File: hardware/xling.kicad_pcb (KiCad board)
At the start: 2 copper layers, 45 x 60 mm, 57 parts, among them J3 MCP73831, J4 USB_OTG, J5 AVR ISP, J6 Battery, Q1 TP0610T, SW2 Up, SW3 Select, SW4 Down, U1 LT1109CZ-12, U2 ATMEGA328P-AU, U3 DEP_128064I, U4 MCP1640B-CH, U5 LM1117-3.3, Y1 8MHz

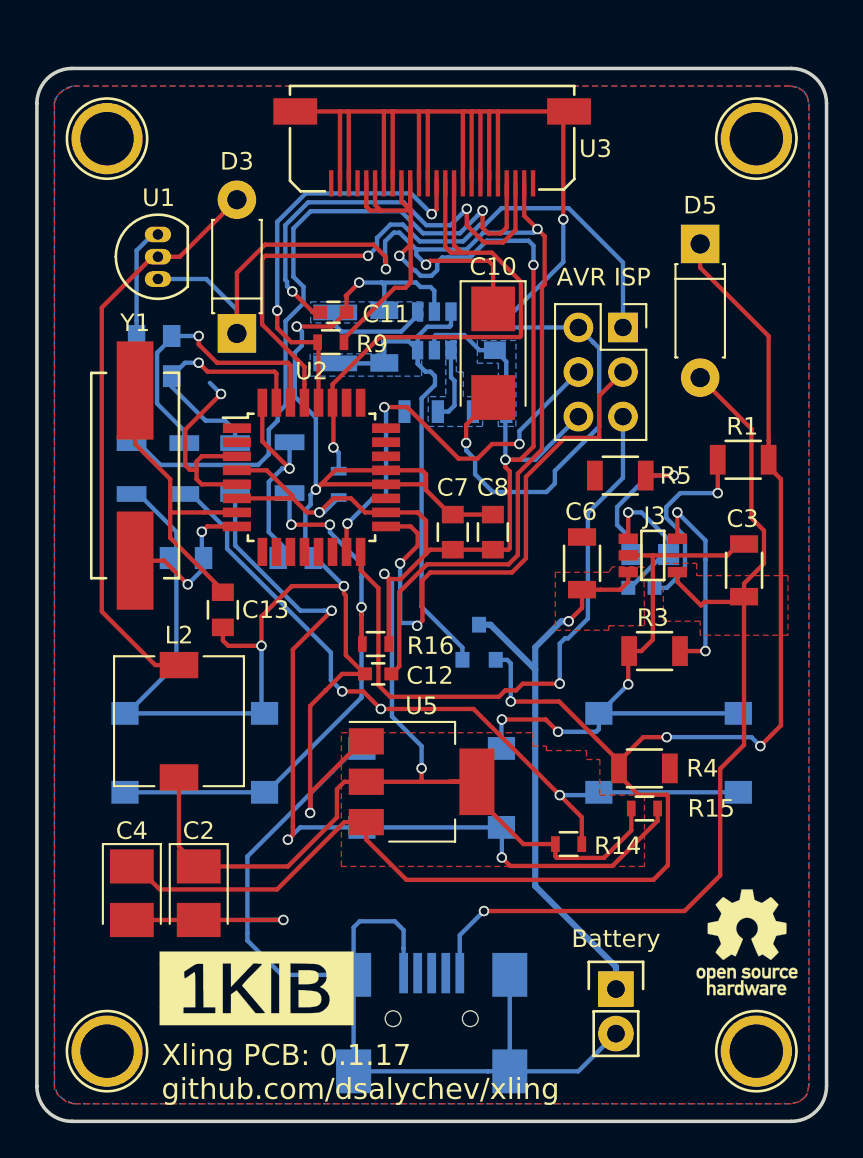
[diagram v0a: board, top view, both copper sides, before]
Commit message: patch 0.1.18: Add new KiCad modules and scheme changes.
Signed-off-by: Dmitry Salychev <darkness.bsd@gmail.com>
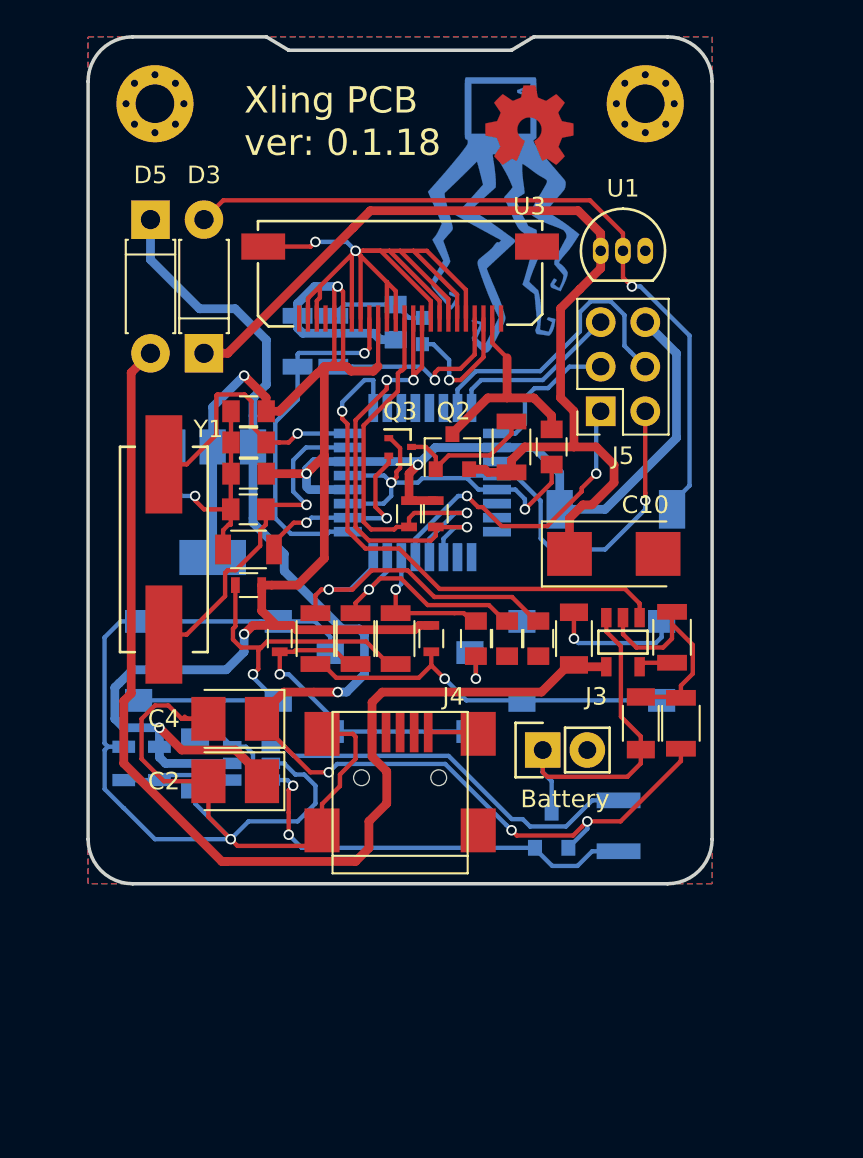
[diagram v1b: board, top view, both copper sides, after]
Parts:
- removed C12: 2.2uF, Capacitors_SMD:C_0603
- removed D1: charging, LEDs:LED_0603
- removed D2: charged, LEDs:LED_0805
- removed the G*** at (131.5, 130.4)
- removed the REF** at (160.0, 134.0)
- removed the REF** at (123.0, 134.0)
- removed the REF** at (160.0, 82.0)
- removed the REF** at (123.0, 82.0)
- removed REF***: OSHW-Logo_5.7x6mm_SilkScreen, Symbols:OSHW-Logo_5.7x6mm_SilkScreen
- added C9: 1pF, Capacitors_SMD:C_0805, F.Cu at (148.3, 99.6)
- added G***: LOGO, Xling Footprints:terterm, B.Cu at (145.5, 86.4)
- added G***: LOGO, Xling Footprints:oshw, F.Cu at (147.1, 81.3)
- added Q2: NTR0202PL, TO_SOT_Packages_SMD:SOT-23, F.Cu at (142.7, 99.8)
- added Q3: NTA4153N, SC-75_SOT-416, F.Cu at (139.7, 99.6)
- added R10: 100K, Resistors_SMD:R_1206, F.Cu at (131.1, 105.4)
- added REF**: MountingHole_2.2mm_M2_Pad_Via, Mounting_Holes:MountingHole_2.2mm_M2_Pad_Via, F.Cu at (125.7, 80.0)
- added REF**: MountingHole_2.2mm_M2_Pad_Via, Mounting_Holes:MountingHole_2.2mm_M2_Pad_Via, F.Cu at (153.7, 80.0)
- C11, L2, U2: moved to B.Cu
- C15, C18, C19, C20, J4, R17, R18, R19, R8: moved to F.Cu
- J6: footprint Pin_Headers:Pin_Header_Straight_1x02 -> Xling Footprints:Pin_Header_Straight_1x02
- R1: value 470R -> 100K; moved to B.Cu
- R5: value 470R -> 100K
- U5: footprint TO_SOT_Packages_SMD:SOT-223-3Lead_TabPin2 -> Xling Footprints:SOT-223-3Lead_TabPin2; moved to B.Cu
- Y1: footprint Crystals:Crystal_HC49-SD_SMD -> Xling Footprints:Crystal_HC49-SD_SMD
- moved L1 32.2 mm to (152.1, 121.2)
- moved D5 31.4 mm to (125.5, 86.6)
- moved L2 27.7 mm to (152.0, 103.1), turned to 0 degrees
- moved R6 27.5 mm to (126.0, 117.6), turned to 270 degrees
- moved U4 26.8 mm to (131.2, 117.6), turned to 180 degrees
- moved SW2 26.7 mm to (128.8, 111.8)
- moved C5 26.6 mm to (128.0, 117.6), turned to 270 degrees
- moved R1 26.3 mm to (133.9, 93.5), turned to 270 degrees
- moved R7 26.3 mm to (124.0, 117.6), turned to 90 degrees
- moved U1 25.3 mm to (151.1, 88.4), turned to 0 degrees
- moved C18 25.2 mm to (144.0, 110.5), turned to 270 degrees
- moved C19 25.1 mm to (145.8, 110.5), turned to 270 degrees
- moved R14 23.5 mm to (131.1, 107.4), turned to 180 degrees
- moved SW4 23.2 mm to (150.6, 111.8)
- moved R15 22.9 mm to (132.8, 110.5), turned to 270 degrees
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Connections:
- J3 pad 1: Net-(D1-Pad1) -> /BAT_STAT
- J4 pad 2: Net-(J4-Pad2) -> (no net)
- J4 pad 3: Net-(J4-Pad3) -> (no net)
- J4 pad 4: Net-(J4-Pad4) -> (no net)
- R1 pad 1: Net-(C4-Pad1) -> +3V3
- R1 pad 2: Net-(D1-Pad2) -> /OLED_RES
- R5 pad 1: GND -> +12V
- U2 pad 1: Net-(U2-Pad1) -> /OLED_RES
- U2 pad 10: Net-(U2-Pad10) -> (no net)
- U2 pad 11: Net-(U2-Pad11) -> (no net)
- U2 pad 12: Net-(U2-Pad12) -> (no net)
- U2 pad 13: Net-(U2-Pad13) -> (no net)
- U2 pad 14: Net-(U2-Pad14) -> (no net)
- U2 pad 19: Net-(U2-Pad19) -> (no net)
- U2 pad 2: Net-(U2-Pad2) -> /OLED_PWR
- U2 pad 22: Net-(U2-Pad22) -> (no net)
- U2 pad 23: Net-(U2-Pad23) -> (no net)
- U2 pad 24: Net-(U2-Pad24) -> (no net)
- U2 pad 25: Net-(U2-Pad25) -> (no net)
- U2 pad 26: Net-(U2-Pad26) -> (no net)
- U2 pad 9: Net-(U2-Pad9) -> /BAT_STAT
- U3 pad 1: Net-(U3-Pad1) -> (no net)
- U3 pad 23: +12V -> /OLED_VCC
- U3 pad 24: Net-(U3-Pad24) -> (no net)
- U3 pad 4: Net-(U3-Pad4) -> (no net)
- U3 pad 9: +3V3 -> /OLED_RES
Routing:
- net GND: track 328.7 -> 220.6 mm, vias 13 -> 9
- net Net-(R15-Pad2): track 49.3 -> 18.7 mm, vias 3 -> 1
- net /BAT_STAT: track 0.00 -> 30.5 mm, vias 0 -> 1
- net Net-(R2-Pad2): track 39.9 -> 11.3 mm
- net /ISP_PDO_MISO: track 35.7 -> 10.0 mm, vias 1 -> 0
- net /ISP_SCK: track 31.7 -> 8.35 mm, vias 2 -> 0
- net Net-(C4-Pad1): track 94.6 -> 72.3 mm, vias 3 -> 4
- net /OLED_RES: track 0.00 -> 20.4 mm, vias 0 -> 1
- net /ISP_RST: track 37.1 -> 18.1 mm, vias 1 -> 2
- net Net-(R14-Pad2): track 43.6 -> 25.3 mm, vias 3 -> 1
- net +12V: track 74.3 -> 56.1 mm, vias 3 -> 0
- net Net-(C11-Pad1): track 24.9 -> 7.74 mm, vias 2 -> 1
- net Net-(L1-Pad2): track 6.25 -> 22.3 mm
- net Net-(C6-Pad1): track 33.6 -> 20.2 mm, vias 1 -> 0
- net /OLED_VCC: track 0.00 -> 12.6 mm
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- removed copper zone on B.Cu, net +3V3
- removed copper zone on F.Cu, net +3V3
- removed copper zone on F.Cu, net Net-(C3-Pad1)
- removed copper zone on B.Cu, net Net-(C5-Pad1)
- removed copper zone on F.Cu, net Net-(C6-Pad1)
- removed copper zone on B.Cu, net Net-(L1-Pad2)
- removed copper zone on B.Cu, net Net-(R6-Pad2)
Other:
- board size 45 x 60 mm -> 35.6 x 48.3 mm
- board text added: "Xling PCB ver: 0.1.18"
- board text added: "terterm.com"
- board text removed: "AVR ISP"
- board text removed: "Battery"
- board text removed: "Down"
- board text removed: "Select"
- board text removed: "Up"
- board text removed: "Xling PCB: 0.1.17 github.com/dsalychev/xling"
- board text removed: "charged"
- board text removed: "charging"
